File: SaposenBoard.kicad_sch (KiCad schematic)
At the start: 64 parts, among them IC1 BSO220, IC2 BSO220, IC3 BSO220, IC4 BSO220, J1 Extra2ch+LED, J2 I2C, J3 Encoder1, J4 Encoder2, J5 ADC4ch, J6 Battery, J7 Motor1, J8 Motor2, Q2 BSS138, SW1 BatterySW, SW2 SW_Push, SW3 SW_Push, U1 NUCLEO-F303K8, U2 A4955GLPTR-T, U3 MPU-6500, U4 A4955GLPTR-T

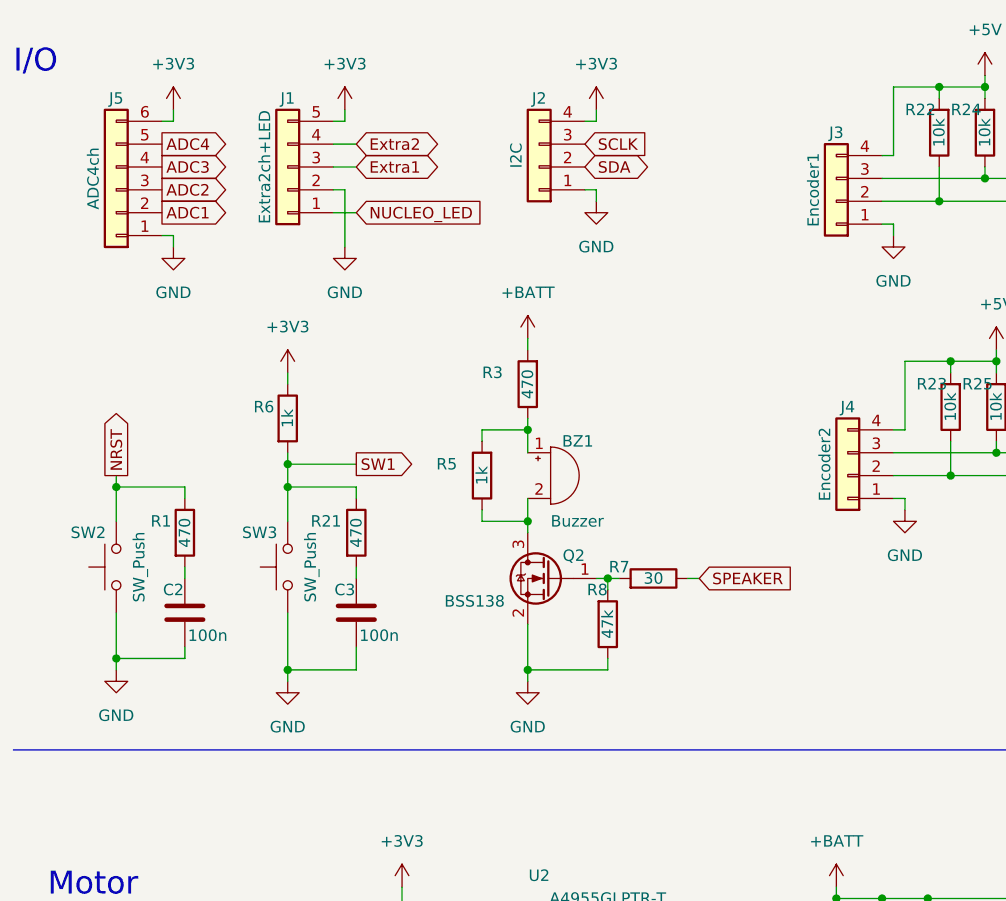
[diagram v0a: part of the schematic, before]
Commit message: [fix]シルク整えた
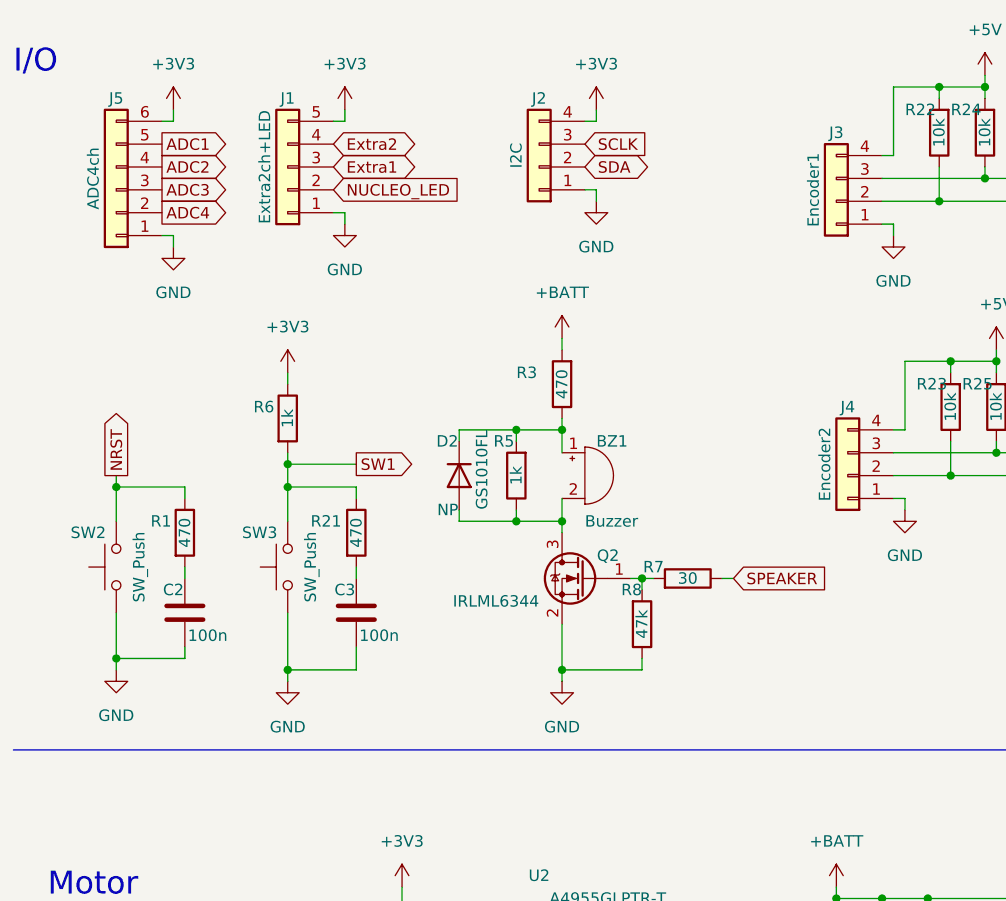
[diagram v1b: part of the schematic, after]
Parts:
- added D2: GS1010FL, Diode_SMD:D_SOD-123F, symbol Device:D
- Q2: value BSS138 -> IRLML6344
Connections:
- net ADC1: now also J5.5 (Pin_5); no longer J5.2 (Pin_2)
- net ADC2: now also J5.4 (Pin_4); no longer J5.3 (Pin_3)
- net ADC3: now also J5.3 (Pin_3); no longer J5.4 (Pin_4)
- net ADC4: now also J5.2 (Pin_2); no longer J5.5 (Pin_5)
- net GND: now also J1.1 (Pin_1); no longer J1.2 (Pin_2)
- net NUCLEO_LED: now also J1.2 (Pin_2); no longer J1.1 (Pin_1)
- net at BZ1.1 (-), R3.1, R5.2: now also D2.1 (K)
- net at BZ1.2 (+), Q2.3 (D), R5.1: now also D2.2 (A)
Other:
- moved on the sheet: BZ1, Q2, R3, R5, R7, R8
